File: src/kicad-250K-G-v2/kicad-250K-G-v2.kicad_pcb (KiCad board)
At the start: 2 copper layers, 35.6 x 47.6 mm, 28 parts, among them P1 In, P2 Out, P3 Power, U1 TL072

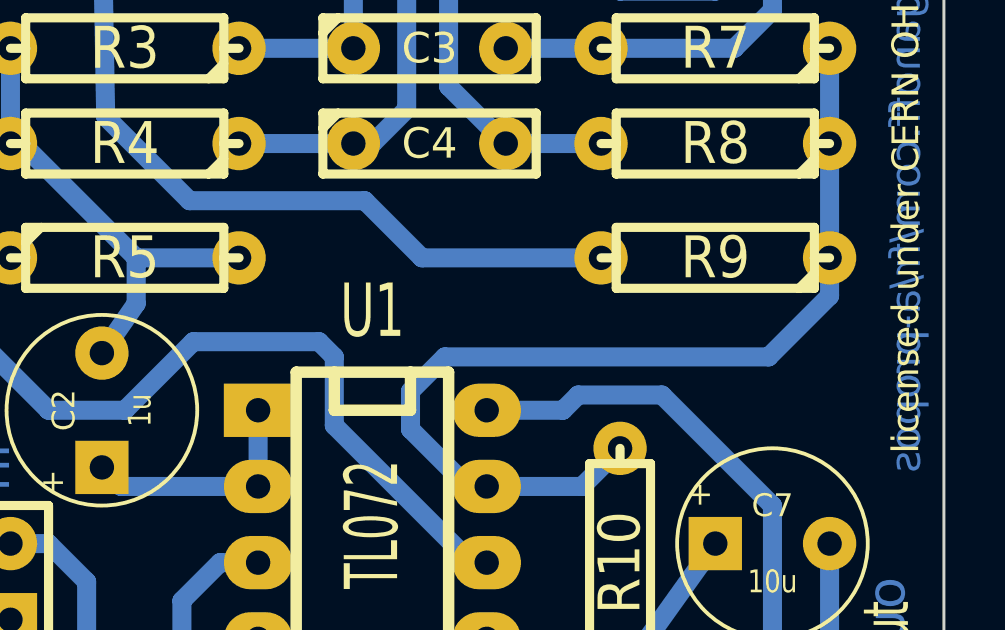
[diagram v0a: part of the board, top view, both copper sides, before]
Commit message: final 2014-07-01
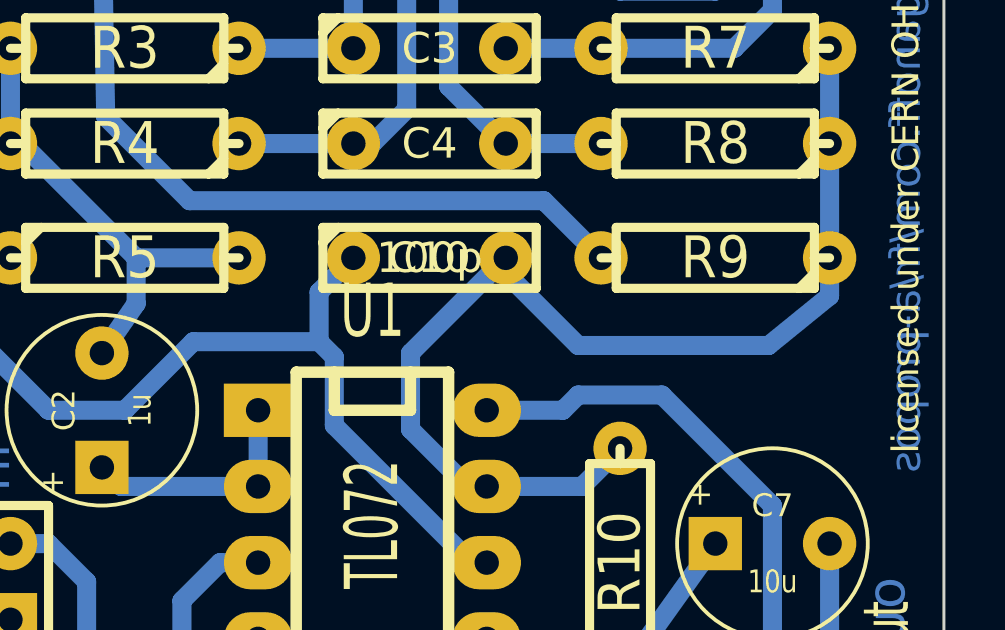
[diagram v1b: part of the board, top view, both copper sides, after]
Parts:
- added C10: 100p, Custom:C2-LARGE_PADS, F.Cu at (130.8, 97.2)
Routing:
- net Net-(C10-Pad2): track 33.1 -> 36.5 mm
- net Net-(C10-Pad1): track 95.5 -> 98.7 mm
